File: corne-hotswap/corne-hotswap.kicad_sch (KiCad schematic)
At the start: 56 parts, among them J1 Battery Connector, J2 nice!view, J3 OLED display, SW1 SW_Push, SW10 SW_Push, SW11 SW_Push, SW12 SW_Push, SW13 SW_Push, SW14 SW_Push, SW15 SW_Push, SW16 SW_Push, SW17 SW_Push, SW18 SW_Push, SW19 SW_Push, SW2 SW_Push, SW20 SW_Push, SW21 SW_Push, SW3 SW_Push, SW4 SW_Push, SW5 SW_Push, SW6 SW_Push, SW7 SW_Push, SW8 SW_Push, SW9 SW_Push, U1 ProMicro

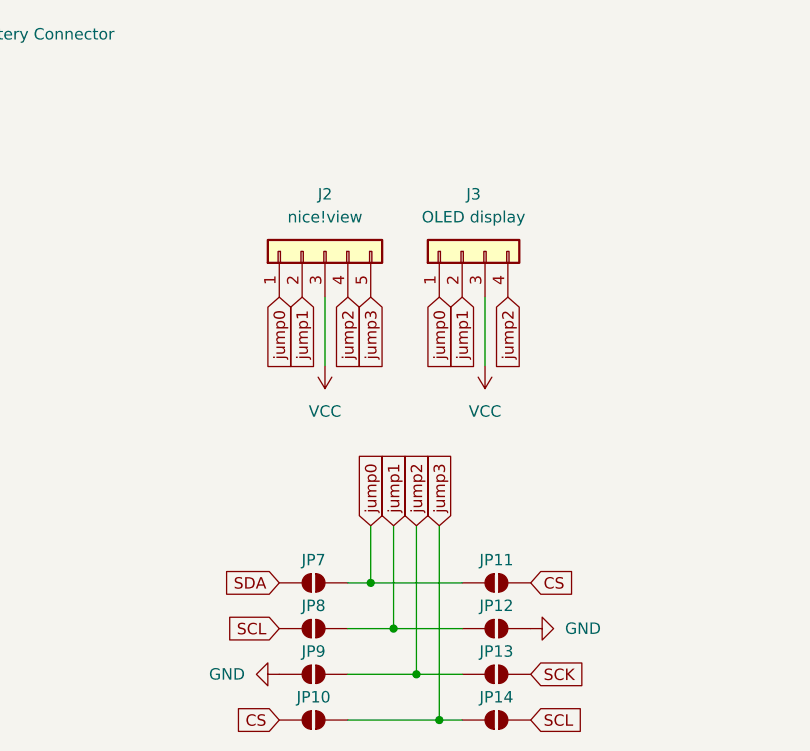
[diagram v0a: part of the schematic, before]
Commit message: update
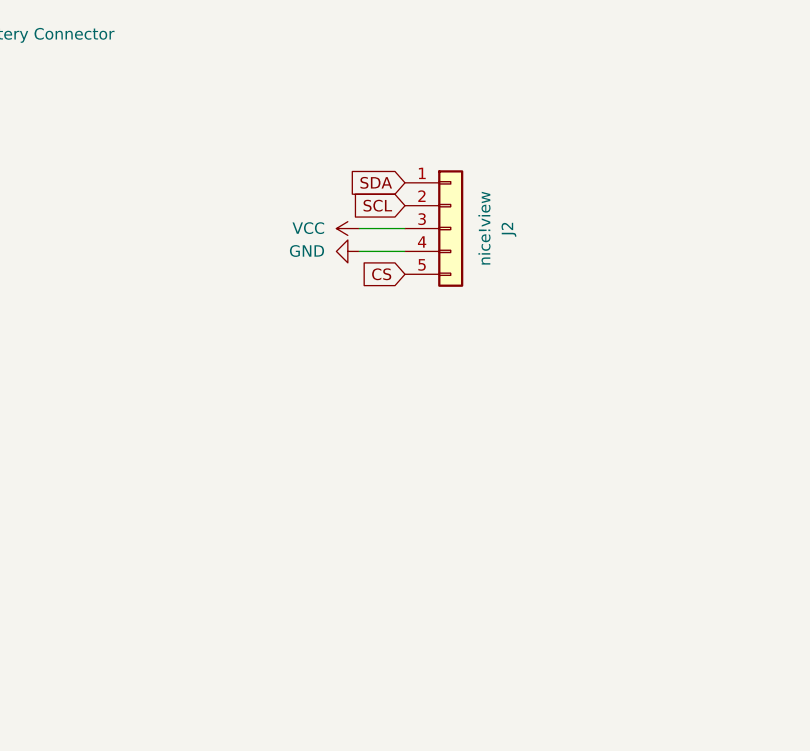
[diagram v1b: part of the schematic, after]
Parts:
- removed J3: OLED display, Project:OLED_Display, symbol Connector_Generic:Conn_01x04
- removed JP10, JP11, JP12, JP13, JP14, JP7, JP8, JP9: SolderJumper_2_Open, Jumper:SolderJumper-2_P1.3mm_Open_RoundedPad1.0x1.5mm, symbol Jumper:SolderJumper_2_Open
- D1, D10, D11, D12, D13, D14, D15, D16, D17, D18, D19, D2, D20, D21, D3, D4, D5, D6, D7, D8, D9: footprint Project:Diode-Reversible -> Project:D_SOD-123F-Reversible
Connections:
- net jump0 is gone; now on net SDA: J2.1 (Pin_1)
- net jump1 is gone; now on net SCL: J2.2 (Pin_2)
- net jump2 is gone; now on net GND: J2.4 (Pin_4)
- net jump3 is gone; now on net CS: J2.5 (Pin_5)
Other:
- moved on the sheet: J2

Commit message: edit
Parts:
- D1, D10, D11, D12, D13, D14, D15, D16, D17, D18, D19, D2, D20, D21, D3, D4, D5, D6, D7, D8, D9: footprint Project:D_SOD-123F-Reversible -> Project:D_SOD-123F-Reversible-Hotswap
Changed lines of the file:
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@@
 			)
 		)
-		(property "Footprint" "Project:D_SOD-123F-Reversible"
+		(property "Footprint" "Project:D_SOD-123F-Reversible-Hotswap"
 			(at 232.41 102.87 0)
 			(effects
@@
 			)
 		)
-		(property "Footprint" "Project:D_SOD-123F-Reversible"
+		(property "Footprint" "Project:D_SOD-123F-Reversible-Hotswap"
 			(at 214.63 120.65 0)
 			(effects
@@
 			)
 		)
-		(property "Footprint" "Project:D_SOD-123F-Reversible"
+		(property "Footprint" "Project:D_SOD-123F-Reversible-Hotswap"
 			(at 250.19 156.21 0)
 			(effects
@@
 			)
 		)
-		(property "Footprint" "Project:D_SOD-123F-Reversible"
+		(property "Footprint" "Project:D_SOD-123F-Reversible-Hotswap"
 			(at 214.63 138.43 0)
 			(effects
@@
 			)
 		)
-		(property "Footprint" "Project:D_SOD-123F-Reversible"
+		(property "Footprint" "Project:D_SOD-123F-Reversible-Hotswap"
 			(at 196.85 120.65 0)
 			(effects
@@
 			)
 		)
-		(property "Footprint" "Project:D_SOD-123F-Reversible"
+		(property "Footprint" "Project:D_SOD-123F-Reversible-Hotswap"
 			(at 179.07 102.87 0)
 			(effects
@@
 			)
 		)
-		(property "Footprint" "Project:D_SOD-123F-Reversible"
+		(property "Footprint" "Project:D_SOD-123F-Reversible-Hotswap"
 			(at 179.07 138.43 0)
 			(effects
@@
 			)
 		)
-		(property "Footprint" "Project:D_SOD-123F-Reversible"
+		(property "Footprint" "Project:D_SOD-123F-Reversible-Hotswap"
 			(at 179.07 120.65 0)
 			(effects
@@
 			)
 		)
-		(property "Footprint" "Project:D_SOD-123F-Reversible"
+		(property "Footprint" "Project:D_SOD-123F-Reversible-Hotswap"
 			(at 196.85 102.87 0)
 			(effects
@@
 			)
 		)
-		(property "Footprint" "Project:D_SOD-123F-Reversible"
+		(property "Footprint" "Project:D_SOD-123F-Reversible-Hotswap"
 			(at 267.97 102.87 0)
 			(effects
@@
 			)
 		)
-		(property "Footprint" "Project:D_SOD-123F-Reversible"
+		(property "Footprint" "Project:D_SOD-123F-Reversible-Hotswap"
 			(at 267.97 138.43 0)
 			(effects
@@
 			)
 		)
-		(property "Footprint" "Project:D_SOD-123F-Reversible"
+		(property "Footprint" "Project:D_SOD-123F-Reversible-Hotswap"
 			(at 214.63 102.87 0)
 			(effects
@@
 			)
 		)
-		(property "Footprint" "Project:D_SOD-123F-Reversible"
+		(property "Footprint" "Project:D_SOD-123F-Reversible-Hotswap"
 			(at 267.97 156.21 0)
 			(effects
@@
 			)
 		)
-		(property "Footprint" "Project:D_SOD-123F-Reversible"
+		(property "Footprint" "Project:D_SOD-123F-Reversible-Hotswap"
 			(at 232.41 120.65 0)
 			(effects
@@
 			)
 		)
-		(property "Footprint" "Project:D_SOD-123F-Reversible"
+		(property "Footprint" "Project:D_SOD-123F-Reversible-Hotswap"
 			(at 250.19 138.43 0)
 			(effects
@@
 			)
 		)
-		(property "Footprint" "Project:D_SOD-123F-Reversible"
+		(property "Footprint" "Project:D_SOD-123F-Reversible-Hotswap"
 			(at 232.41 156.21 0)
 			(effects
@@
 			)
 		)
-		(property "Footprint" "Project:D_SOD-123F-Reversible"
+		(property "Footprint" "Project:D_SOD-123F-Reversible-Hotswap"
 			(at 267.97 120.65 0)
 			(effects
@@
 			)
 		)
-		(property "Footprint" "Project:D_SOD-123F-Reversible"
+		(property "Footprint" "Project:D_SOD-123F-Reversible-Hotswap"
 			(at 196.85 138.43 0)
 			(effects
@@
 			)
 		)
-		(property "Footprint" "Project:D_SOD-123F-Reversible"
+		(property "Footprint" "Project:D_SOD-123F-Reversible-Hotswap"
 			(at 250.19 102.87 0)
 			(effects
@@
 			)
 		)
-		(property "Footprint" "Project:D_SOD-123F-Reversible"
+		(property "Footprint" "Project:D_SOD-123F-Reversible-Hotswap"
 			(at 250.19 120.65 0)
 			(effects
@@
 			)
 		)
-		(property "Footprint" "Project:D_SOD-123F-Reversible"
+		(property "Footprint" "Project:D_SOD-123F-Reversible-Hotswap"
 			(at 232.41 138.43 0)
 			(effects
